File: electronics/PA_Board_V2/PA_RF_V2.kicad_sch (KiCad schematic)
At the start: 80 parts, among them J1 Conn_Coaxial, J5 Conn_Coaxial, J7 Conn_Coaxial, J8 Conn_Coaxial, K1 G6E, Q2 BC848W, U1 PSA4-5043+, U14 Directional_Coupler, U3 PSA4-5043+, U4 RA35H1516M, U8 TPS22810DBV

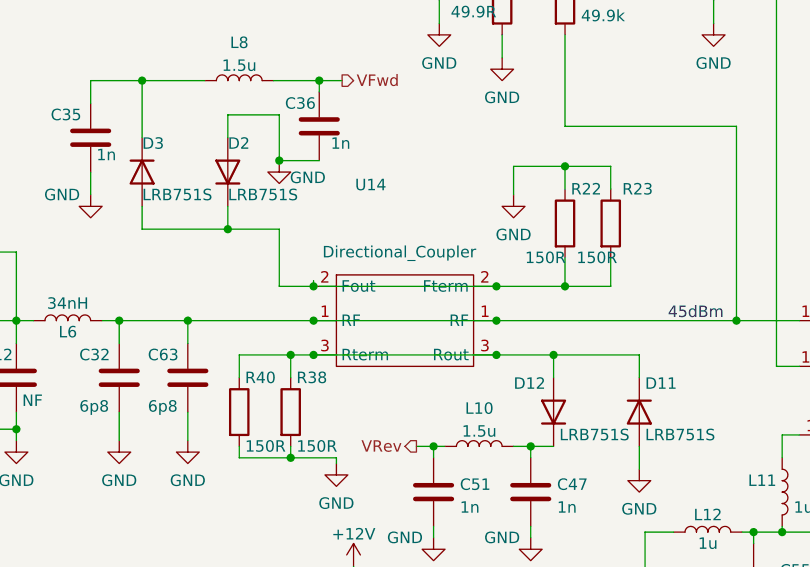
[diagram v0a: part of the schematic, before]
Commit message: Save unlocked Kicad files for PA Board V2
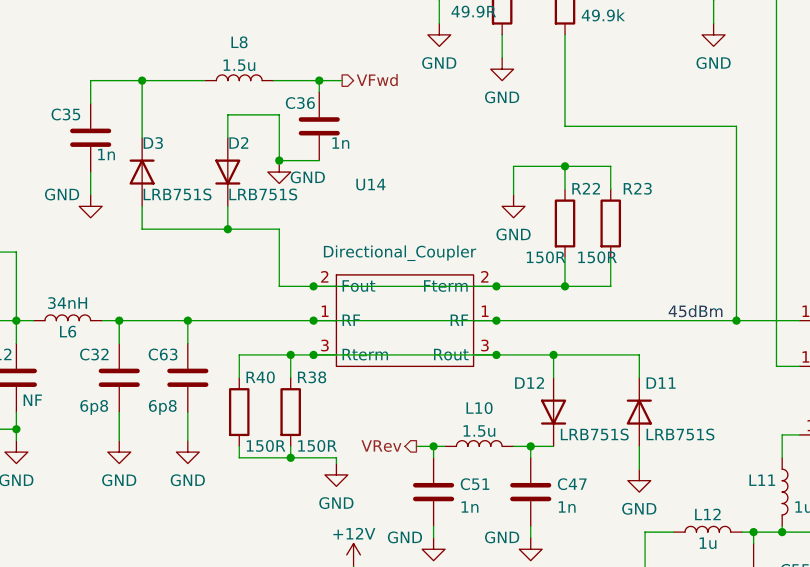
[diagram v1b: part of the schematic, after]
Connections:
- net at R22.2, R23.2, U14.2 (Fterm): now also D2.1 (K), D3.2 (A)
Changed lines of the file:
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@@
-    (stroke (width 0) (type default))
-  )
-  (wire (pts (xy 197.485 98.425) (xy 197.485 99.06))
     (stroke (width 0) (type default))
   )
@@
     (stroke (width 0) (type default))
   )
-  (wire (pts (xy 198.12 99.06) (xy 217.805 99.06))
-    (stroke (width 0) (type default))
-  )
   (wire (pts (xy 142.875 95.25) (xy 144.145 95.25))
     (stroke (width 0) (type default))
@@
     (stroke (width 0) (type default))
   )
+  (wire (pts (xy 197.485 99.06) (xy 217.805 99.06))
+    (stroke (width 0) (type default))
+  )
